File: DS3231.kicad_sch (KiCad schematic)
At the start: 8 parts, among them IC1 DS3231, J1 Conn_01x08_Pin

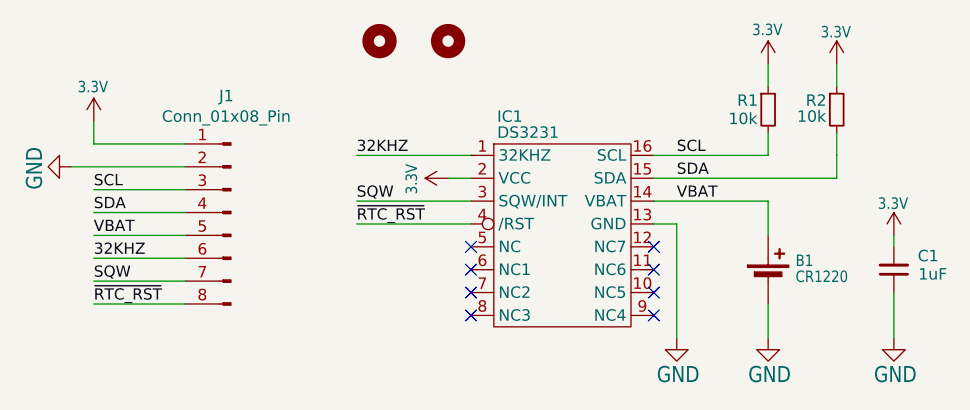
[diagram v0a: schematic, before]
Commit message: updated routing + symbol update
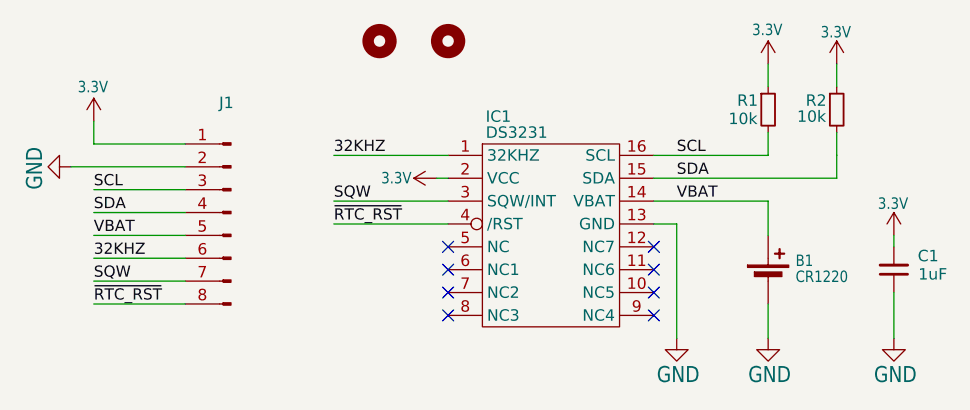
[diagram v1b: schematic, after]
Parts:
- B1: now left out of the parts list
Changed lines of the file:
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@@
 	)
 	(no_connect
-		(at 151.13 107.95)
+		(at 148.59 107.95)
 	)
 	(no_connect
@@
 	)
 	(no_connect
-		(at 151.13 110.49)
+		(at 148.59 110.49)
 	)
 	(no_connect
-		(at 151.13 105.41)
+		(at 148.59 105.41)
 	)
 	(no_connect
@@
 	)
 	(no_connect
-		(at 151.13 102.87)
+		(at 148.59 102.87)
 	)
 	(no_connect
@@
 	(wire
 		(pts
-			(xy 138.43 100.33) (xy 151.13 100.33)
+			(xy 135.89 100.33) (xy 148.59 100.33)
 		)
 		(stroke
@@
 	(wire
 		(pts
-			(xy 138.43 92.71) (xy 151.13 92.71)
+			(xy 135.89 92.71) (xy 148.59 92.71)
 		)
 		(stroke
@@
 	(wire
 		(pts
-			(xy 148.59 95.25) (xy 151.13 95.25)
+			(xy 147.32 95.25) (xy 148.59 95.25)
 		)
 		(stroke
@@
 	(wire
 		(pts
-			(xy 138.43 97.79) (xy 151.13 97.79)
+			(xy 135.89 97.79) (xy 148.59 97.79)
 		)
 		(stroke
@@
 	)
 	(label "SQW"
-		(at 138.43 97.79 0)
+		(at 135.89 97.79 0)
 		(fields_autoplaced yes)
 		(effects
@@
 	)
 	(label "32KHZ"
-		(at 138.43 92.71 0)
+		(at 135.89 92.71 0)
 		(fields_autoplaced yes)
 		(effects
@@
 	)
 	(label "~{RTC_RST}"
-		(at 138.43 100.33 0)
+		(at 135.89 100.33 0)
 		(fields_autoplaced yes)
 		(effects
@@
 	(symbol
 		(lib_id "power:+3.3V")
-		(at 148.59 95.25 90)
+		(at 147.32 95.25 90)
 		(unit 1)
 		(exclude_from_sim no)
@@
 		(dnp no)
 		(property "Reference" "#U$02"
-			(at 148.59 95.25 0)
+			(at 147.32 95.25 0)
 			(effects
 				(font
@@
 		)
 		(property "Value" "3.3V"
-			(at 145.288 97.028 0)
+			(at 144.526 94.488 90)
 			(effects
 				(font
@@
 		)
 		(property "Footprint" ""
-			(at 148.59 95.25 0)
+			(at 147.32 95.25 0)
 			(effects
 				(font
@@
 		)
 		(property "Datasheet" ""
-			(at 148.59 95.25 0)
+			(at 147.32 95.25 0)
 			(effects
 				(font
@@
 		)
 		(property "Description" "Power symbol creates a global label with name \"+3.3V\""
-			(at 148.59 95.25 0)
+			(at 147.32 95.25 0)
 			(effects
 				(font
@@
 		(unit 1)
 		(exclude_from_sim no)
-		(in_bom yes)
+		(in_bom no)
 		(on_board yes)
 		(dnp no)
@@
 				(path "/3054a26c-491b-4a2c-bd9e-2e89ff40ccf1"
 					(reference "B1")
+					(unit 1)
+				)
+			)
+		)
+	)
+	(symbol
+		(lib_id "external_library:DS3231")
+		(at 152.4 111.76 0)
+		(unit 1)
+		(exclude_from_sim no)
+		(in_bom yes)
+		(on_board yes)
+		(dnp no)
+		(property "Reference" "IC1"
+			(at 154.178 88.392 0)
+			(effects
+				(font
+					(size 1.27 1.27)
+				)
+			)
+		)
+		(property "Value" "DS3231"
+			(at 156.21 90.17 0)
+			(effects
+				(font
+					(size 1.27 1.27)
+				)
+			)
+		)
+		(property "Footprint" "Package_SO:SOIC-16W_7.5x10.3mm_P1.27mm"
+			(at 162.306 114.808 0)
+			(effects
+				(font
+					(size 1.27 1.27)
+				)
+				(hide yes)
+			)
+		)
+		(property "Datasheet" ""
+			(at 149.86 92.71 0)
+			(effects
+				(font
+					(size 1.27 1.27)
+				)
+				(hide yes)
+			)
+		)
+		(property "Description" "IC RTC CLK/CALENDAR I2C 16SOIC"
+			(at 149.86 92.71 0)
+			(effects
+				(font
+					(size 1.27 1.27)
+				)
+				(hide yes)
+			)
+		)
+		(property "Manufacturer" "Analog Devices Inc./Maxim Integrated"
+			(at 152.4 111.76 0)
+			(effects
+				(font
+					(size 1.27 1.27)
+				)
+				(hide yes)
+			)
+		)
+		(property "MPN" "DS3231M+TRL"
+			(at 152.4 111.76 0)
+			(effects
+				(font
+					(size 1.27 1.27)
+				)
+				(hide yes)
+			)
+		)
+		(property "Supplier" "DigiKey"
+			(at 152.4 111.76 0)
+			(effects
+				(font
+					(size 1.27 1.27)
+				)
+				(hide yes)
+			)
+		)
+		(property "SPN" "DS3231M+TRLTR-ND - Tape & Reel (TR)"
+			(at 152.4 111.76 0)
+			(effects
+				(font
+					(size 1.27 1.27)
+				)
+				(hide yes)
+			)
+		)
+		(property "Component package type" "/"
+			(at 152.4 111.76 0)
+			(effects
+				(font
+					(size 1.27 1.27)
+				)
+				(hide yes)
+			)
+		)
+		(pin "1"
+		)
+		(pin "10"
+		)
+		(pin "15"
+		)
+		(pin "14"
+		)
+		(pin "5"
+		)
+		(pin "8"
+		)
+		(pin "12"
+		)
+		(pin "7"
+		)
+		(pin "9"
+		)
+		(pin "6"
+		)
+		(pin "2"
+		)
+		(pin "3"
+		)
+		(pin "13"
+		)
+		(pin "11"
+		)
+		(pin "16"
+		)
+		(pin "4"
+		)
+		(instances
+			(project "DS3231"
+				(path "/3054a26c-491b-4a2c-bd9e-2e89ff40ccf1"
+					(reference "IC1")
 					(unit 1)
 				)
@@
 	)
 	(symbol
-		(lib_id "external_library:DS3231")
-		(at 153.67 111.76 0)
-		(unit 1)
-		(exclude_from_sim no)
-		(in_bom yes)
-		(on_board yes)
-		(dnp no)
-		(property "Reference" "IC1"
-			(at 155.448 88.392 0)
-			(effects
-				(font
-					(size 1.27 1.27)
-				)
-			)
-		)
-		(property "Value" "DS3231"
-			(at 157.48 90.17 0)
-			(effects
-				(font
-					(size 1.27 1.27)
-				)
-			)
-		)
-		(property "Footprint" "Package_SO:SOIC-16W_7.5x10.3mm_P1.27mm"
-			(at 163.576 114.808 0)
-			(effects
-				(font
-					(size 1.27 1.27)
-				)
-				(hide yes)
-			)
-		)
-		(property "Datasheet" ""
-			(at 151.13 92.71 0)
-			(effects
-				(font
-					(size 1.27 1.27)
-				)
-				(hide yes)
-			)
-		)
-		(property "Description" "IC RTC CLK/CALENDAR I2C 16SOIC"
-			(at 151.13 92.71 0)
-			(effects
-				(font
-					(size 1.27 1.27)
-				)
-				(hide yes)
-			)
-		)
-		(property "Manufacturer" "Analog Devices Inc./Maxim Integrated"
-			(at 153.67 111.76 0)
-			(effects
-				(font
-					(size 1.27 1.27)
-				)
-				(hide yes)
-			)
-		)
-		(property "MPN" "DS3231M+TRL"
-			(at 153.67 111.76 0)
-			(effects
-				(font
-					(size 1.27 1.27)
-				)
-				(hide yes)
-			)
-		)
-		(property "Supplier" "DigiKey"
-			(at 153.67 111.76 0)
-			(effects
-				(font
-					(size 1.27 1.27)
-				)
-				(hide yes)
-			)
-		)
-		(property "SPN" "DS3231M+TRLTR-ND - Tape & Reel (TR)"
-			(at 153.67 111.76 0)
-			(effects
-				(font
-					(size 1.27 1.27)
-				)
-				(hide yes)
-			)
-		)
-		(property "Component package type" "/"
-			(at 153.67 111.76 0)
-			(effects
-				(font
-					(size 1.27 1.27)
-				)
-				(hide yes)
-			)
-		)
-		(pin "1"
-		)
-		(pin "10"
-		)
-		(pin "15"
-		)
-		(pin "14"
-		)
-		(pin "5"
-		)
-		(pin "8"
-		)
-		(pin "12"
-		)
-		(pin "7"
-		)
-		(pin "9"
-		)
-		(pin "6"
-		)
-		(pin "2"
-		)
-		(pin "3"
-		)
-		(pin "13"
-		)
-		(pin "11"
-		)
-		(pin "16"
-		)
-		(pin "4"
-		)
-		(instances
-			(project "DS3231"
-				(path "/3054a26c-491b-4a2c-bd9e-2e89ff40ccf1"
-					(reference "IC1")
-					(unit 1)
-				)
-			)
-		)
-	)
-	(symbol
 		(lib_id "power:+3.3V")
 		(at 109.22 88.9 0)
@@
 		(dnp no)
 		(property "Reference" "J1"
-			(at 123.952 86.106 0)
+			(at 123.952 86.868 0)
 			(effects
 				(font
@@
 					(size 1.27 1.27)
 				)
-			)
-		)
+				(hide yes)
+			)
+		)
